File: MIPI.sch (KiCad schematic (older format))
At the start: 46 parts, among them J8 ARJP11A-MASA-B-A-EMU2, U1 AllWinner-S3(FBGA-234), Y2 32.768kHz, Y3 24MHz

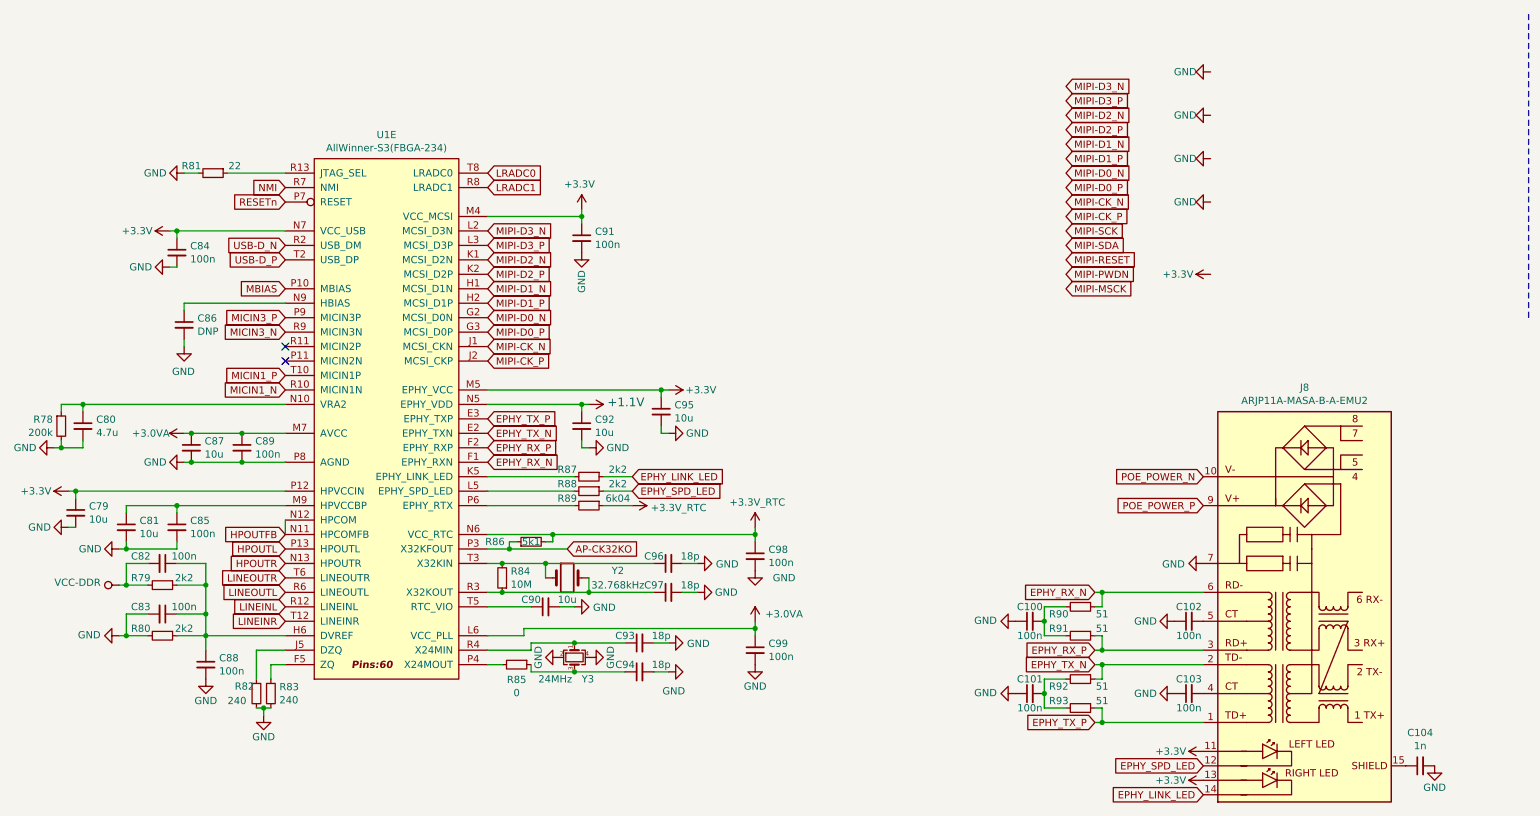
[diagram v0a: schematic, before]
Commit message: update
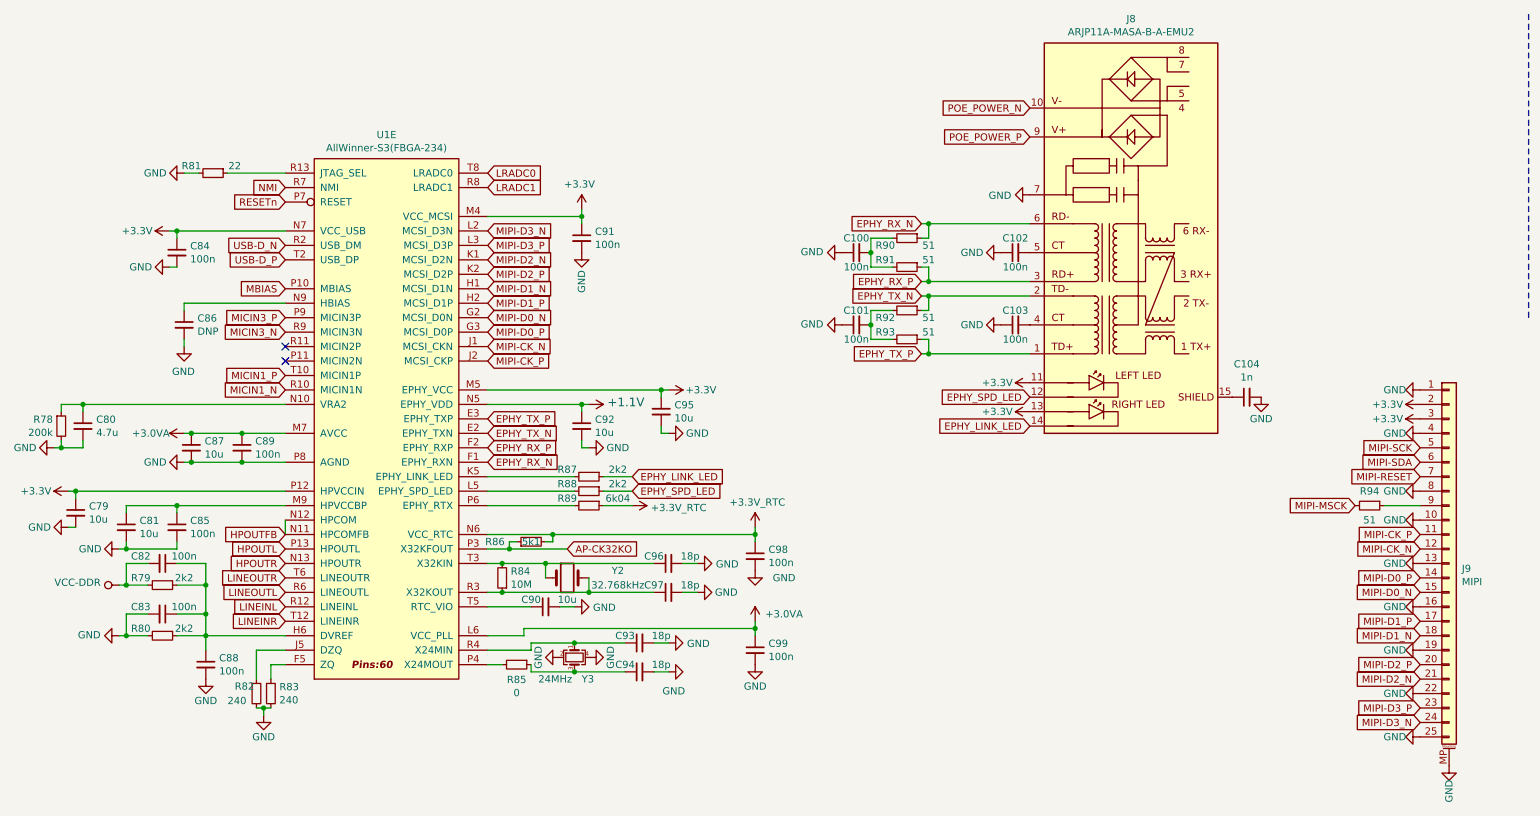
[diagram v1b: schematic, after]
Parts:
- added J9: MIPI, otter:FH35C-25S, symbol Connector_Generic_MountingPin:Conn_01x25_MountingPin
- added R94: 51, otter:C_0402, symbol Device:R_Small
- U1: footprint OLIMEX_IC-FP:FBGA-234(Pitch-0.65mm_Pad-0.3mm_11x11x1.08mm) -> otter:FBGA-234(Pitch-0.65mm_Pad-0.3mm_11x11x1.08mm)
- Y2, Y3: footprint (none) -> otter:Oscillator_3225
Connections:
- net +3V3: now also J9.2 (Pin_2), J9.3 (Pin_3)
- net GND: now also J9.1 (Pin_1), J9.10 (Pin_10), J9.13 (Pin_13), J9.16 (Pin_16), J9.19 (Pin_19), J9.22 (Pin_22), J9.25 (Pin_25), J9.4 (Pin_4), J9.8 (Pin_8), J9.MP (MountPin)
- net MIPI-CK_N: now also J9.12 (Pin_12)
- net MIPI-CK_P: now also J9.11 (Pin_11)
- net MIPI-D0_N: now also J9.15 (Pin_15)
- net MIPI-D0_P: now also J9.14 (Pin_14)
- net MIPI-D1_N: now also J9.18 (Pin_18)
- net MIPI-D1_P: now also J9.17 (Pin_17)
- net MIPI-D2_N: now also J9.21 (Pin_21)
- net MIPI-D2_P: now also J9.20 (Pin_20)
- net MIPI-D3_N: now also J9.24 (Pin_24)
- net MIPI-D3_P: now also J9.23 (Pin_23)
- net MIPI-MSCK: now also R94.2
- net MIPI-RESET: now also J9.7 (Pin_7)
- net MIPI-SCK: now also J9.5 (Pin_5)
- net MIPI-SDA: now also J9.6 (Pin_6)
- new net: J9.9 (Pin_9), R94.1
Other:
- moved on the sheet: C100, C101, C102, C103, C104, J8, R90, R91, R92, R93

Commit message: update
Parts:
- Y2: footprint otter:Oscillator_3225 -> Crystal:Crystal_SMD_3215-2Pin_3.2x1.5mm
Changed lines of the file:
@@
 F 0 "Y2" H 5000 4750 50  0000 C CNN
 F 1 "32.768kHz" H 5000 4650 50  0000 C CNN
-F 2 "otter:Oscillator_3225" H 4650 4700 50  0001 C CNN
+F 2 "Crystal:Crystal_SMD_3215-2Pin_3.2x1.5mm" H 4650 4700 50  0001 C CNN
 F 3 "~" H 4650 4700 50  0001 C CNN
 	1    4650 4700

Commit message: update
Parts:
- Y2: footprint Crystal:Crystal_SMD_3215-2Pin_3.2x1.5mm -> otter:Crystal_SMD_3215-2Pin_3.2x1.5mm
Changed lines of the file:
@@
 F 0 "Y2" H 5000 4750 50  0000 C CNN
 F 1 "32.768kHz" H 5000 4650 50  0000 C CNN
-F 2 "Crystal:Crystal_SMD_3215-2Pin_3.2x1.5mm" H 4650 4700 50  0001 C CNN
+F 2 "otter:Crystal_SMD_3215-2Pin_3.2x1.5mm" H 4650 4700 50  0001 C CNN
 F 3 "~" H 4650 4700 50  0001 C CNN
 	1    4650 4700
